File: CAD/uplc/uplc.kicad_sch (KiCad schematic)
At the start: 33 parts, among them J1 Conn_01x06_Pin, J2 SM12B-GHS-TB(LF)(SN), K1 G6K-2F-Y, K2 G6K-2F-Y, U1 AP63201WU, U2 TBD62003AFWG, U3 ESP32-C3-WROOM-02, Y1 32.568khz 3.2x1.5 12.5pf

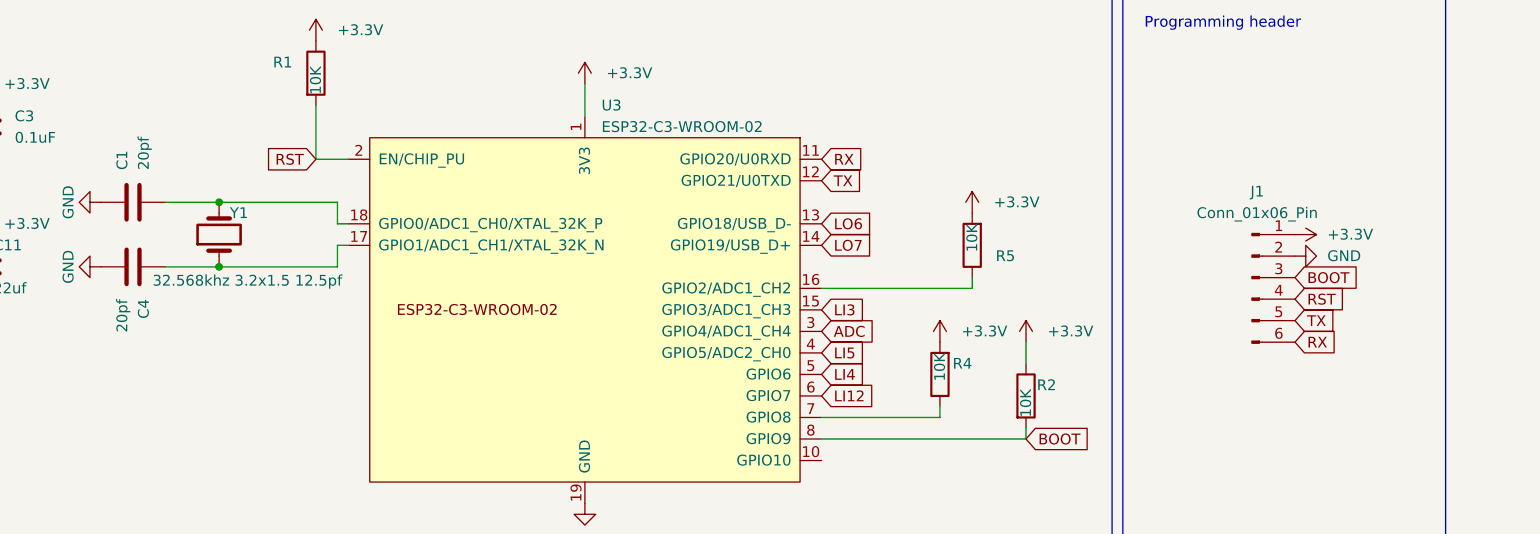
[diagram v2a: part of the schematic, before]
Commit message: Production push rev 1.2
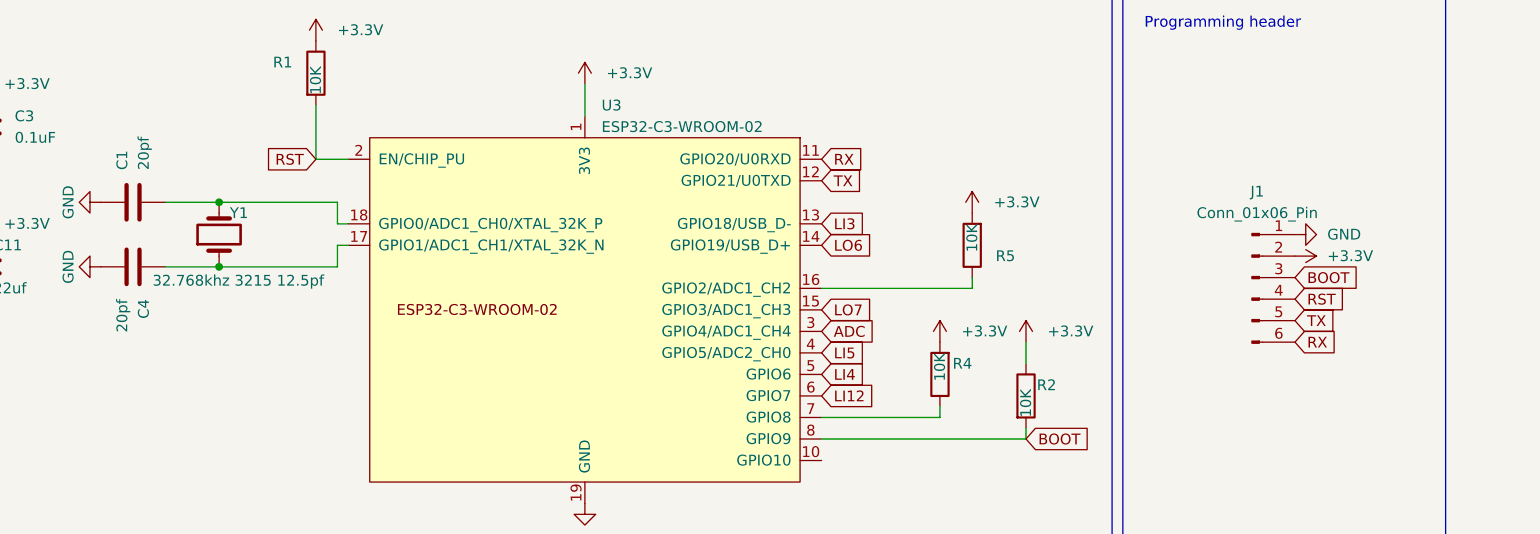
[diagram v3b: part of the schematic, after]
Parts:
- C5: LCSC Part # (none) -> C162422
- J1: LCSC Part # (none) -> DNP
- L1: LCSC Part # (none) -> C98340
- R14: LCSC Part # (none) -> C11481
- R15: LCSC Part # (none) -> C137950
- U1: LCSC Part # (none) -> C2071044
- Y1: value 32.568khz 3.2x1.5 12.5pf -> 32.768khz 3215 12.5pf
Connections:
- net +3.3V: now also J1.2 (Pin_2); no longer J1.1 (Pin_1)
- net GND: now also J1.1 (Pin_1); no longer J1.2 (Pin_2)
- net LI3: now also U3.13 (GPIO18/USB_D-); no longer U3.15 (GPIO3/ADC1_CH3)
- net LO6: now also U3.14 (GPIO19/USB_D+); no longer U3.13 (GPIO18/USB_D-)
- net LO7: now also U3.15 (GPIO3/ADC1_CH3); no longer U3.14 (GPIO19/USB_D+)
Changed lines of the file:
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@@
     )
   )
-  (global_label "LO7" (shape input) (at 120.65 45.72 0) (fields_autoplaced)
-    (effects (font (size 1.27 1.27)) (justify left))
-    (property "Intersheetrefs" "${INTERSHEET_REFS}" (at 129.32 45.72 0)
+  (global_label "LO7" (shape input) (at 120.65 53.34 0) (fields_autoplaced)
+    (effects (font (size 1.27 1.27)) (justify left))
+    (property "Intersheetrefs" "${INTERSHEET_REFS}" (at 129.32 53.34 0)
       (effects (font (size 1.27 1.27)) (justify left) hide)
     )
@@
     )
   )
-  (global_label "LI3" (shape input) (at 120.65 53.34 0) (fields_autoplaced)
-    (effects (font (size 1.27 1.27)) (justify left))
-    (property "Intersheetrefs" "${INTERSHEET_REFS}" (at 130.5295 53.34 0)
+  (global_label "LI3" (shape input) (at 120.65 43.18 0) (fields_autoplaced)
+    (effects (font (size 1.27 1.27)) (justify left))
+    (property "Intersheetrefs" "${INTERSHEET_REFS}" (at 130.5295 43.18 0)
       (effects (font (size 1.27 1.27)) (justify left) hide)
     )
@@
     )
   )
-  (global_label "LO6" (shape input) (at 120.65 43.18 0) (fields_autoplaced)
-    (effects (font (size 1.27 1.27)) (justify left))
-    (property "Intersheetrefs" "${INTERSHEET_REFS}" (at 129.32 43.18 0)
+  (global_label "LO6" (shape input) (at 120.65 45.72 0) (fields_autoplaced)
+    (effects (font (size 1.27 1.27)) (justify left))
+    (property "Intersheetrefs" "${INTERSHEET_REFS}" (at 129.32 45.72 0)
       (effects (font (size 1.27 1.27)) (justify left) hide)
     )
@@
       (effects (font (size 1.27 1.27)) hide)
     )
-    (property "LCSC Part #" "" (at 85.09 125.73 0)
+    (property "LCSC Part #" "C137950" (at 85.09 125.73 0)
       (effects (font (size 1.27 1.27)) hide)
     )
@@
     )
   )
-  (symbol (lib_id "power:+3.3V") (at 176.53 44.45 270) (unit 1)
-    (in_bom yes) (on_board yes) (dnp no) (fields_autoplaced)
-    (property "Reference" "#PWR033" (at 172.72 44.45 0)
-      (effects (font (size 1.27 1.27)) hide)
-    )
-    (property "Value" "+3.3V" (at 180.34 44.45 90)
-      (effects (font (size 1.27 1.27)) (justify left))
-    )
-    (property "Footprint" "" (at 176.53 44.45 0)
-      (effects (font (size 1.27 1.27)) hide)
-    )
-    (property "Datasheet" "" (at 176.53 44.45 0)
+  (symbol (lib_id "power:+3.3V") (at 176.53 46.99 270) (unit 1)
+    (in_bom yes) (on_board yes) (dnp no) (fields_autoplaced)
+    (property "Reference" "#PWR033" (at 172.72 46.99 0)
+      (effects (font (size 1.27 1.27)) hide)
+    )
+    (property "Value" "+3.3V" (at 180.34 46.99 90)
+      (effects (font (size 1.27 1.27)) (justify left))
+    )
+    (property "Footprint" "" (at 176.53 46.99 0)
+      (effects (font (size 1.27 1.27)) hide)
+    )
+    (property "Datasheet" "" (at 176.53 46.99 0)
       (effects (font (size 1.27 1.27)) hide)
     )
@@
       (effects (font (size 1.27 1.27)))
     )
+    (property "LCSC Part #" "C98340" (at 73.66 113.03 0)
+      (effects (font (size 1.27 1.27)) hide)
+    )
     (pin "1")
     (pin "2")
@@
     )
     (property "Datasheet" "https://www.diodes.com/assets/Datasheets/AP63200-AP63201-AP63203-AP63205.pdf" (at 48.26 115.57 0)
+      (effects (font (size 1.27 1.27)) hide)
+    )
+    (property "LCSC Part #" "C2071044" (at 48.26 115.57 0)
       (effects (font (size 1.27 1.27)) hide)
     )
@@
     )
   )
-  (symbol (lib_id "power:GND") (at 176.53 46.99 90) (unit 1)
-    (in_bom yes) (on_board yes) (dnp no)
-    (property "Reference" "#PWR034" (at 182.88 46.99 0)
-      (effects (font (size 1.27 1.27)) hide)
-    )
-    (property "Value" "GND" (at 180.34 46.99 90)
+  (symbol (lib_id "power:GND") (at 176.53 44.45 90) (unit 1)
+    (in_bom yes) (on_board yes) (dnp no)
+    (property "Reference" "#PWR034" (at 182.88 44.45 0)
+      (effects (font (size 1.27 1.27)) hide)
+    )
+    (property "Value" "GND" (at 180.34 44.45 90)
       (effects (font (size 1.27 1.27)) (justify right))
     )
-    (property "Footprint" "" (at 176.53 46.99 0)
-      (effects (font (size 1.27 1.27)) hide)
-    )
-    (property "Datasheet" "" (at 176.53 46.99 0)
+    (property "Footprint" "" (at 176.53 44.45 0)
+      (effects (font (size 1.27 1.27)) hide)
+    )
+    (property "Datasheet" "" (at 176.53 44.45 0)
       (effects (font (size 1.27 1.27)) hide)
     )
@@
       (effects (font (size 1.27 1.27)) hide)
     )
-    (property "LCSC Part #" "" (at 171.45 49.53 0)
+    (property "LCSC Part #" "DNP" (at 171.45 49.53 0)
       (effects (font (size 1.27 1.27)) hide)
     )
@@
       (effects (font (size 1.27 1.27)) hide)
     )
-    (property "LCSC Part #" "" (at 22.86 116.84 0)
+    (property "LCSC Part #" "C162422" (at 22.86 116.84 0)
       (effects (font (size 1.27 1.27)) hide)
     )
@@
       (effects (font (size 1.27 1.27)) (justify right))
     )
-    (property "Value" "32.568khz 3.2x1.5 12.5pf" (at 41.667 49.8894 90)
+    (property "Value" "32.768khz 3215 12.5pf" (at 41.667 49.8894 90)
       (effects (font (size 1.27 1.27)) (justify right))
     )
@@
       (effects (font (size 1.27 1.27)) hide)
     )
-    (property "Datasheet" "~" (at 49.53 44.45 0)
+    (property "Datasheet" "https://datasheet.lcsc.com/lcsc/1810171817_Seiko-Epson-Q13FC1350000400_C32346.pdf" (at 49.53 44.45 0)
       (effects (font (size 1.27 1.27)) hide)
     )
@@
       (effects (font (size 1.27 1.27)) hide)
     )
-    (property "LCSC Part #" "" (at 85.09 116.84 0)
-      (effects (font (size 1.27 1.27)) hide)
-    )
+    (property "LCSC Part #" "C11481" (at 85.09 116.84 0)
+      (effects (font (size 1.27 1.27)) hide)
+    )
